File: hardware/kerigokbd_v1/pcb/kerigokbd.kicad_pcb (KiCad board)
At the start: 2 copper layers, 139.5 x 92 mm, 83 parts, among them J1 USB4520-03-0-A, J2 I2C, J3 SWD, J4 SJ-3501-SMT-TR, SW1 Key_SW, SW10 Key_SW, SW11 Key_SW, SW12 Key_SW, SW13 Key_SW, SW14 Key_SW, SW15 Key_SW, SW16 Key_SW, SW17 Key_SW, SW18 Key_SW, SW19 Key_SW, SW2 Key_SW, SW20 Key_SW, SW21 Key_SW, SW22 Key_SW, SW23 Key_SW, SW24 Key_SW, SW3 Key_SW, SW4 Key_SW, SW5 Key_SW, SW6 Key_SW, SW7 Key_SW, SW8 Key_SW, SW9 Key_SW, U1 TLV75533PDBVR, U2 RP2040, U3 W25Q16JVUXIQ, Y1 12MHz

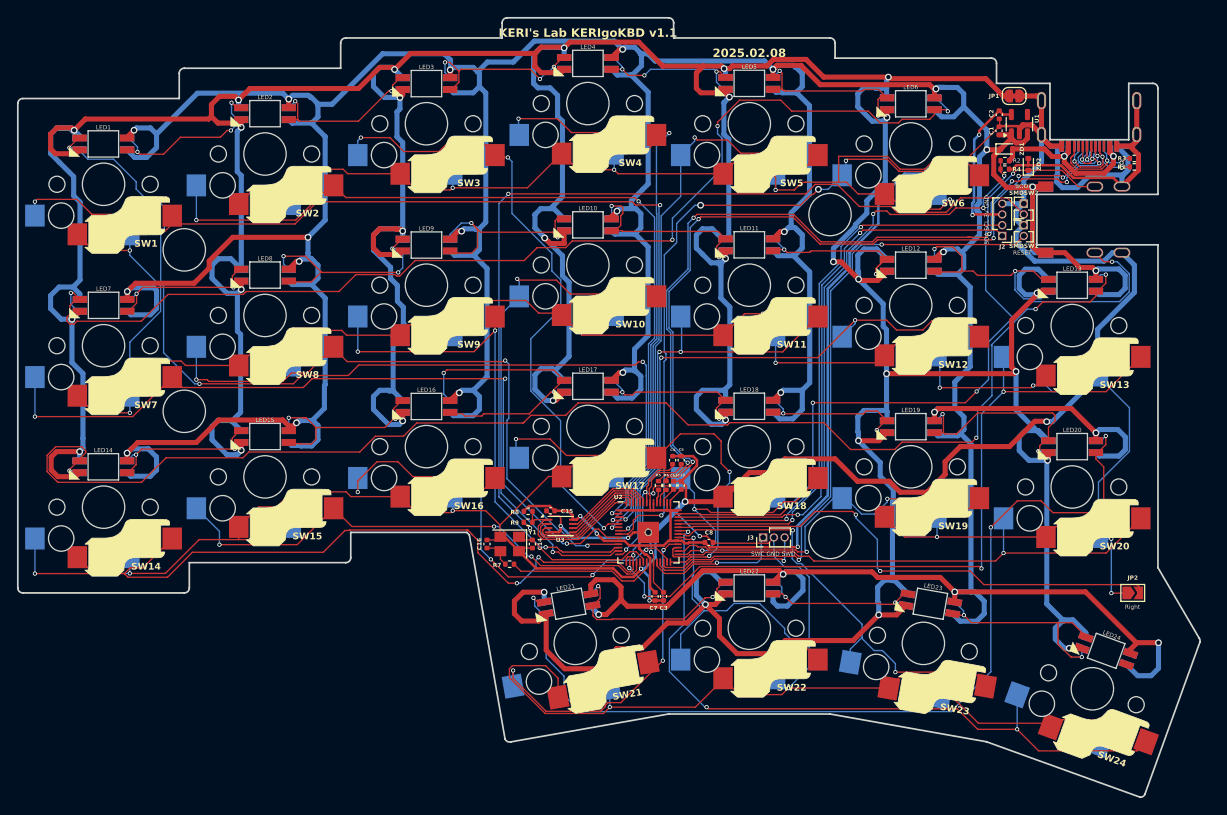
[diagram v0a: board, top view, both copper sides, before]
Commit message: update PCB v2026.02.22a
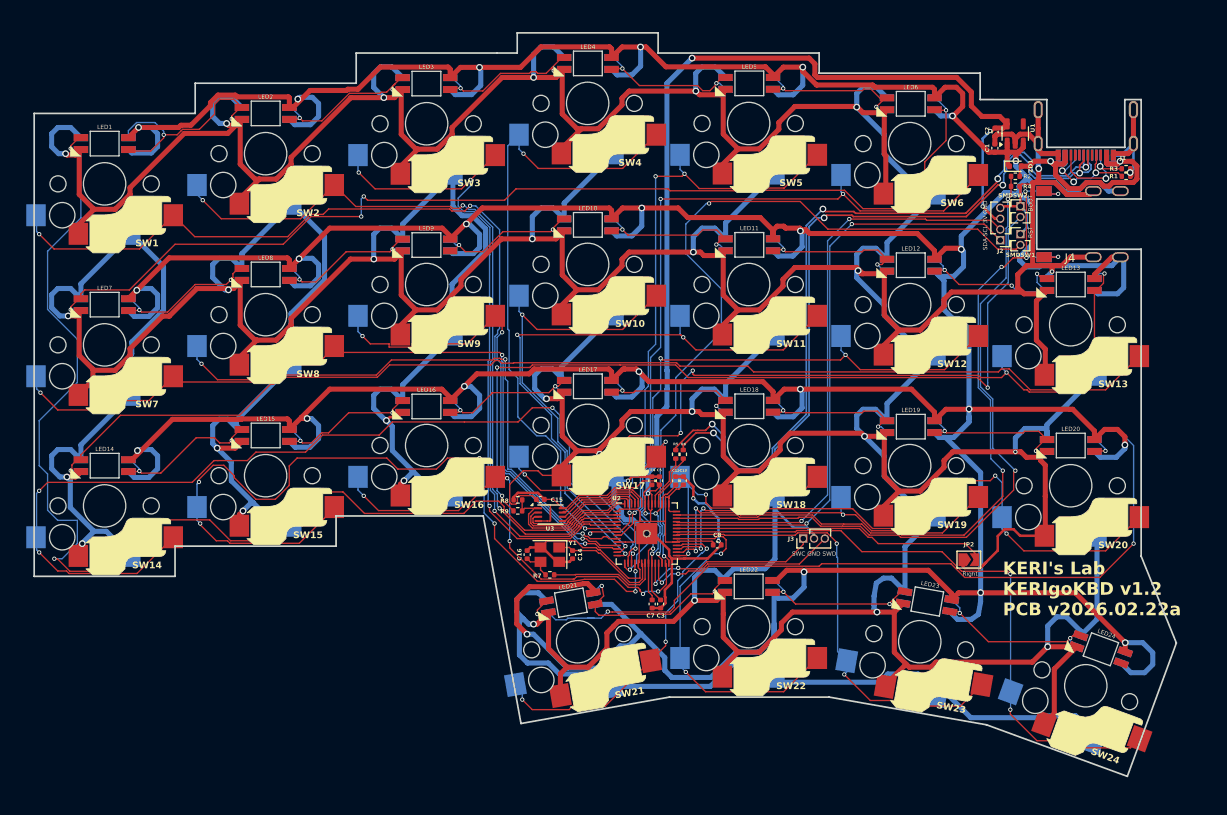
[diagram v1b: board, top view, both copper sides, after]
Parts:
- removed JP1: LED_EN, Jumper:SolderJumper-2_P1.3mm_Bridged_RoundedPad1.0x1.5mm
- removed ZD2: NSR0520V2T5G, Diode_SMD:D_SOD-523
- J1: moved to F.Cu
- J4: footprint kbd_local:PJ-398A-5A_PJ-399B-6A-dual -> kbd_local:SJ-3501-SMT-TR-dual; moved to F.Cu
- moved JP2 19.7 mm to (128.0, 79.1)
- moved C14 4.91 mm to (81.2, 78.5)
- moved C16 4.91 mm to (75.8, 78.5)
- moved R7 4.91 mm to (78.5, 80.9)
- moved Y1 4.91 mm to (78.5, 78.5)
- moved J3 4.74 mm to (108.4, 76.6)
- moved R5 4.20 mm to (93.4, 66.7)
- moved R6 4.20 mm to (94.3, 66.7)
- moved C5 3.54 mm to (91.4, 69.8)
- moved C4 3.45 mm to (90.6, 69.8)
- moved R4 2.38 mm to (133.5, 35.0)
- moved ZD1 2.29 mm to (133.5, 32.7)
- moved R2 2.22 mm to (133.5, 33.8)
- moved C1 2.10 mm to (131.0, 30.5)
- moved C2 2.10 mm to (131.1, 28.6)
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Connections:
- J1 pad B6: /D+ -> unconnected-(J1-D+-PadB6)
- J1 pad B7: /D- -> unconnected-(J1-D--PadB7)
- J4 pad R: /SERIAL -> GND
- J4 pad S: GND -> +5V
- J4 pad T: +5V -> /SERIAL
- LED1 pad 3: /LED_GND -> GND
- LED10 pad 3: /LED_GND -> GND
- LED11 pad 3: /LED_GND -> GND
- LED12 pad 3: /LED_GND -> GND
- LED13 pad 3: /LED_GND -> GND
- LED14 pad 3: /LED_GND -> GND
- LED15 pad 3: /LED_GND -> GND
- LED16 pad 3: /LED_GND -> GND
- LED17 pad 3: /LED_GND -> GND
- LED18 pad 3: /LED_GND -> GND
- LED19 pad 3: /LED_GND -> GND
- LED2 pad 3: /LED_GND -> GND
- LED20 pad 3: /LED_GND -> GND
- LED21 pad 3: /LED_GND -> GND
- LED22 pad 3: /LED_GND -> GND
- LED23 pad 3: /LED_GND -> GND
- LED24 pad 3: /LED_GND -> GND
- LED3 pad 3: /LED_GND -> GND
- LED4 pad 3: /LED_GND -> GND
- LED5 pad 3: /LED_GND -> GND
- LED6 pad 3: /LED_GND -> GND
- LED7 pad 3: /LED_GND -> GND
- LED8 pad 3: /LED_GND -> GND
- LED9 pad 3: /LED_GND -> GND
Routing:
- net /LED_GND: track 730.4 -> 0.00 mm, vias 31 -> 0
- net GND: track 863.2 -> 1400.1 mm, vias 36 -> 33
- net +3V3: track 144.3 -> 182.6 mm
- net /KEY15: track 60.8 -> 97.1 mm, vias 3 -> 6
- net +5V: track 722.5 -> 750.4 mm, vias 27 -> 24
- net /LED: track 113.6 -> 141.0 mm, vias 4 -> 2
- net /SPLIT_HAND: track 61.8 -> 37.2 mm, vias 2 -> 0
- net /KEY14: track 91.5 -> 113.5 mm, vias 3 -> 4
- net /KEY11: track 50.8 -> 72.7 mm
- net Net-(LED16-DOUT): track 35.2 -> 18.4 mm
- net /SERIAL: track 109.9 -> 93.6 mm, vias 5 -> 6
- net Net-(LED13-DOUT): track 159.8 -> 144.4 mm, vias 4 -> 2
- net /D+: track 103.7 -> 89.0 mm, vias 8 -> 4
- net /KEY17: track 50.1 -> 37.5 mm
- net Net-(U2-RUN): track 77.0 -> 88.4 mm
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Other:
- board size 139.5 x 92 mm -> 134.8 x 87.7 mm
- board text added: "KERI's Lab KERIgoKBD v1.2 PCB v2026.02.22a"
- board text added: "RST"
- board text removed: "2025.02.08"
- board text removed: "KERI's Lab KERIgoKBD v1.1"
- board text removed: "RESET"
